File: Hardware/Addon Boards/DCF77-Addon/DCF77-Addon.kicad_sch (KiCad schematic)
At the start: 16 parts, among them J1 Misc-PortD, J2 Addon_Conn, J4 Misc-PortA, J5 I2C, J6 ST-Link, J8 VDD, U1 HPP845E031R1, U2 DCF77-Module

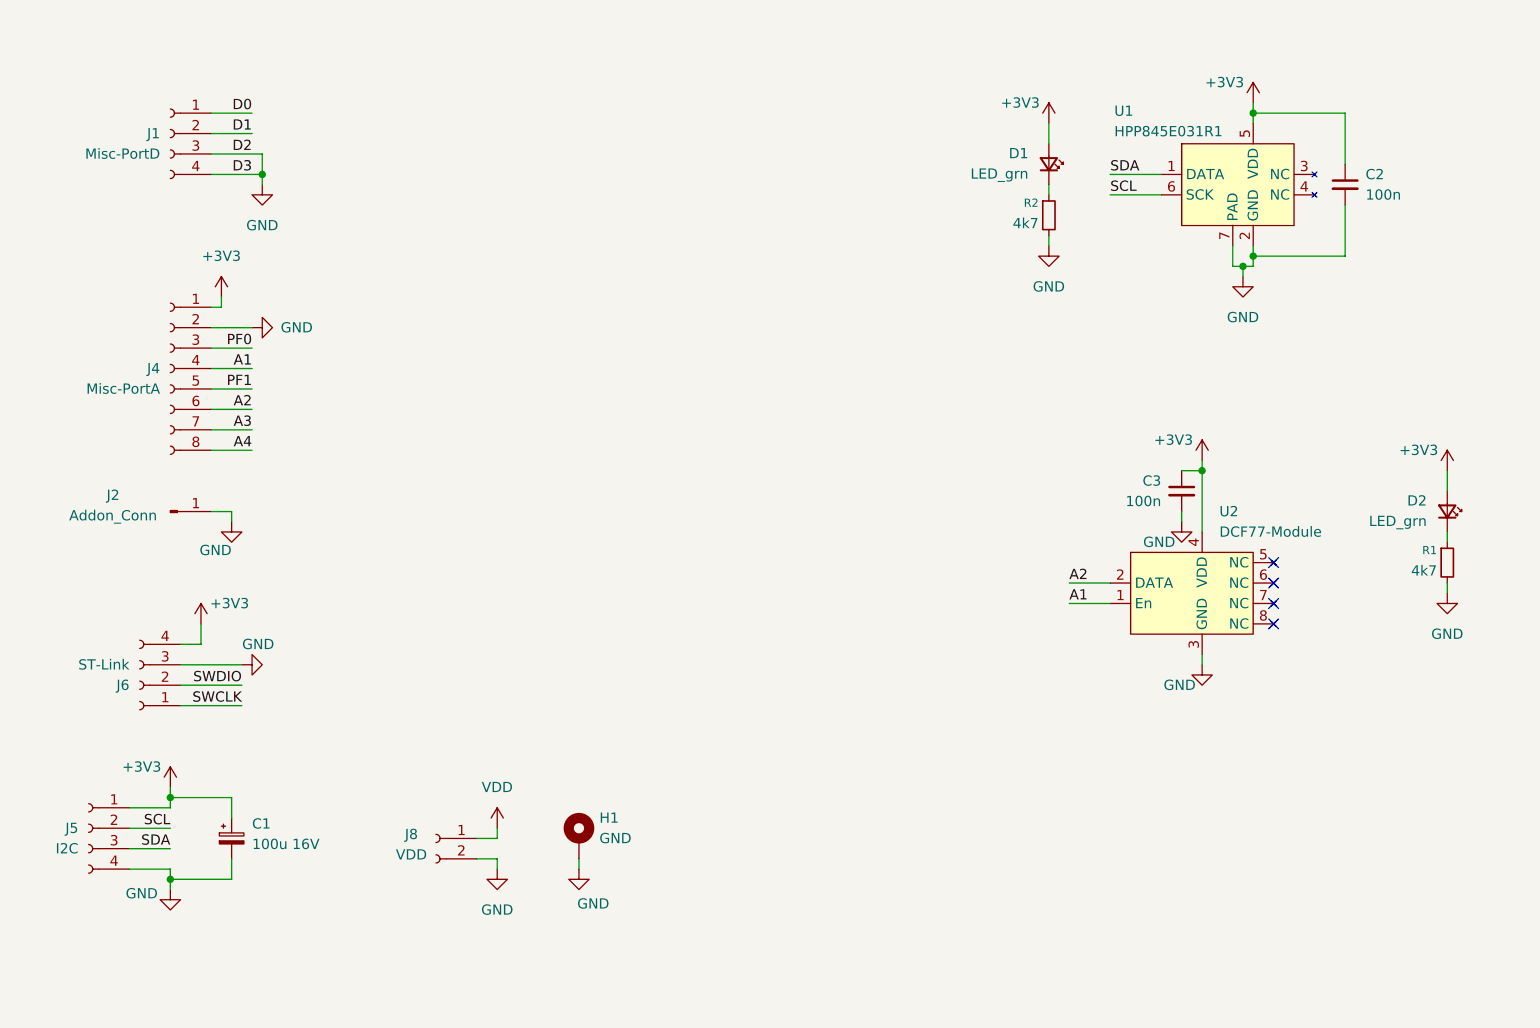
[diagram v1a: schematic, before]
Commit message: cleanup of project data and files
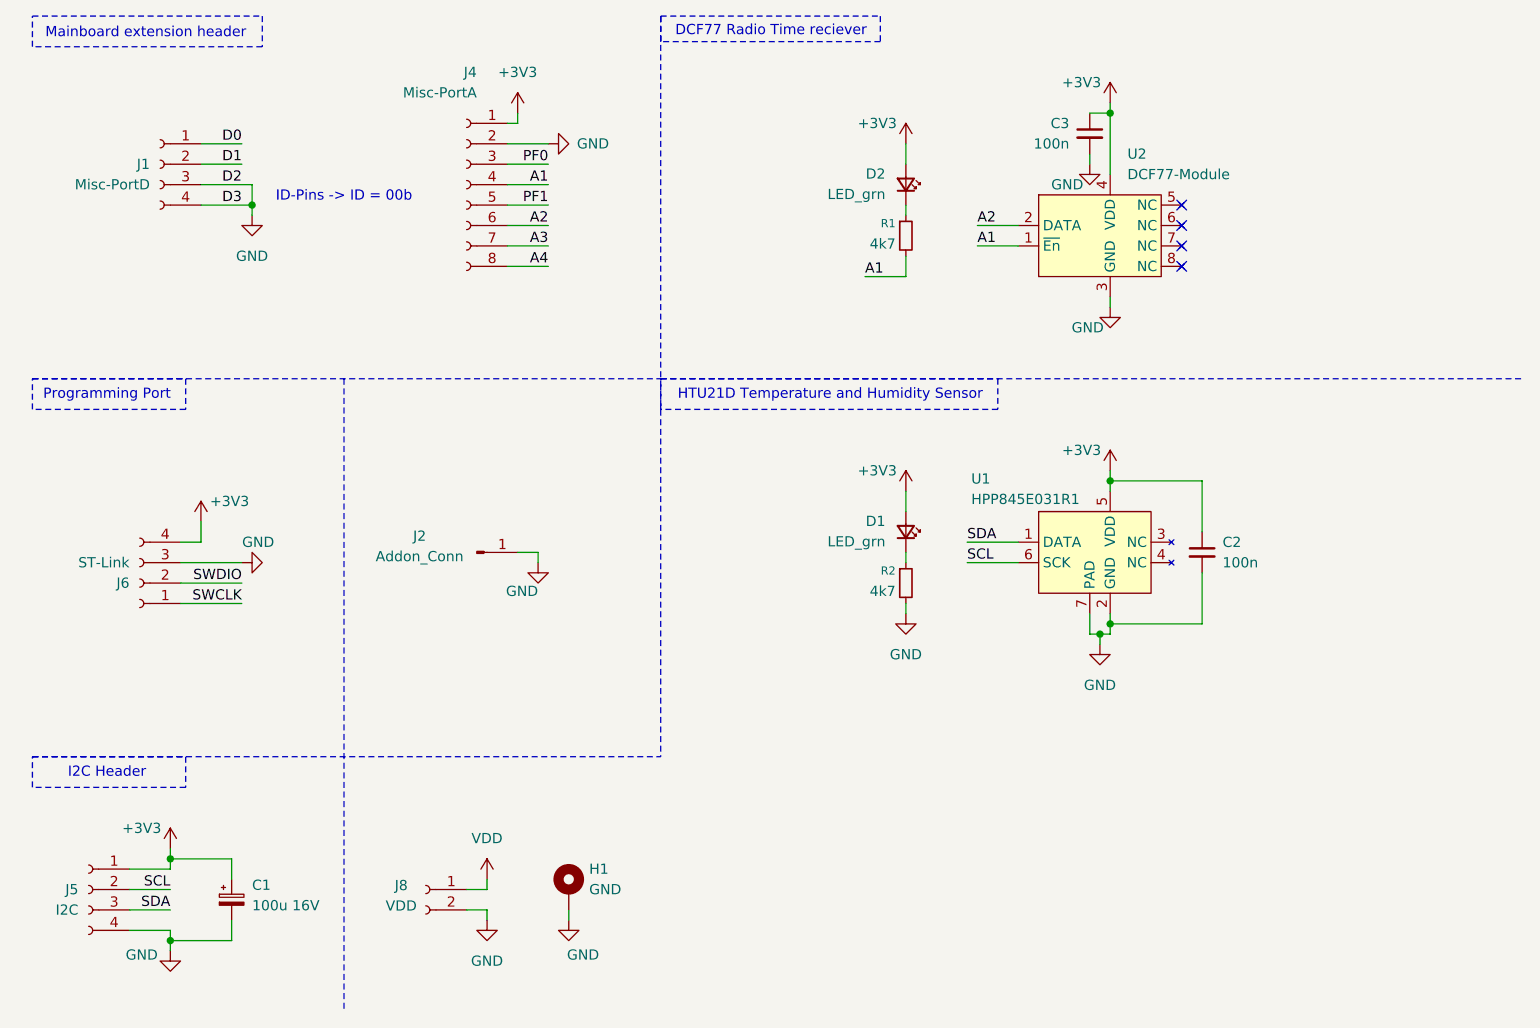
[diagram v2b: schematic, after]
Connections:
- net A1: now also R1.2
- net GND: no longer R1.2
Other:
- note added: "DCF77 Radio Time reciever"
- note added: "HTU21D Temperature and Humidity Sensor"
- note added: "I2C Header"
- note added: "ID-Pins -> ID = 00b"
- note added: "Mainboard extension header"
- note added: "Programming Port"
- moved on the sheet: C1, C2, C3, D1, D2, H1, J1, J2, J4, J5, J6, J8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
